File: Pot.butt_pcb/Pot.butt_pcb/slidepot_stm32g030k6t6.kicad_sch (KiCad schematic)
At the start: 11 parts, among them J3 Conn_01x05_Male, SW10 SW_Push, U2 STM32G030K6T6

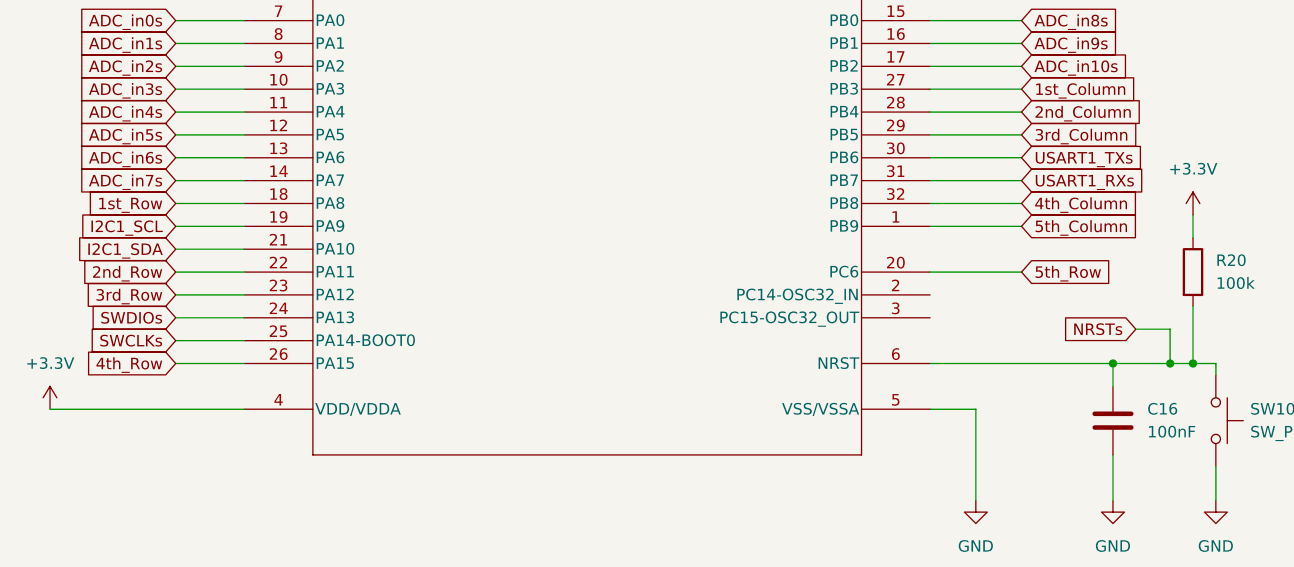
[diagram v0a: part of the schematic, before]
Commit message: Pot.but_pcb in progress
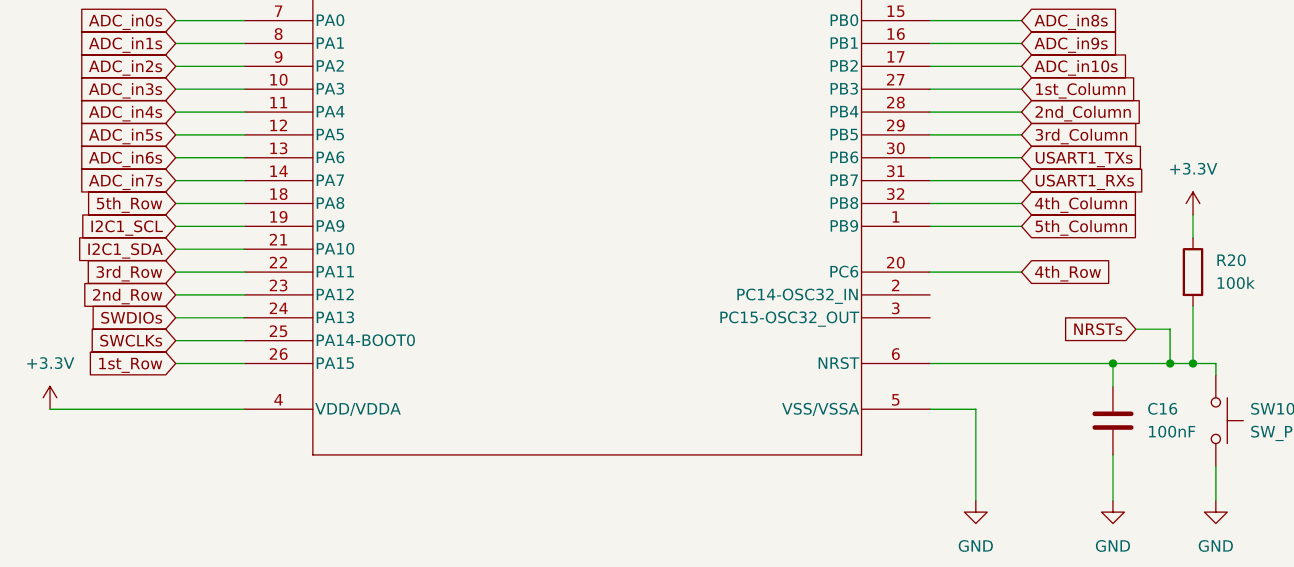
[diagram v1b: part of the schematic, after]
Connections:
- net 1st_Row: now also U2.26 (PA15); no longer U2.18 (PA8)
- net 2nd_Row: now also U2.23 (PA12); no longer U2.22 (PA11)
- net 3rd_Row: now also U2.22 (PA11); no longer U2.23 (PA12)
- net 4th_Row: now also U2.20 (PC6); no longer U2.26 (PA15)
- net 5th_Row: now also U2.18 (PA8); no longer U2.20 (PC6)
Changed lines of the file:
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@@
     )
   )
-  (global_label "4th_Row" (shape input) (at 49.53 83.82 180) (fields_autoplaced)
+  (global_label "1st_Row" (shape input) (at 49.53 83.82 180) (fields_autoplaced)
     (effects (font (size 1.27 1.27)) (justify right))
-    (property "Intersheet References" "${INTERSHEET_REFS}" (id 0) (at 39.3155 83.7406 0)
+    (property "Intersheet References" "${INTERSHEET_REFS}" (id 0) (at 39.4364 83.7406 0)
       (effects (font (size 1.27 1.27)) (justify right) hide)
     )
@@
     )
   )
-  (global_label "2nd_Row" (shape input) (at 49.53 73.66 180) (fields_autoplaced)
+  (global_label "3rd_Row" (shape input) (at 49.53 73.66 180) (fields_autoplaced)
     (effects (font (size 1.27 1.27)) (justify right))
-    (property "Intersheet References" "${INTERSHEET_REFS}" (id 0) (at 38.8921 73.5806 0)
+    (property "Intersheet References" "${INTERSHEET_REFS}" (id 0) (at 39.255 73.5806 0)
       (effects (font (size 1.27 1.27)) (justify right) hide)
     )
@@
     )
   )
-  (global_label "1st_Row" (shape input) (at 49.53 66.04 180) (fields_autoplaced)
+  (global_label "5th_Row" (shape input) (at 49.53 66.04 180) (fields_autoplaced)
     (effects (font (size 1.27 1.27)) (justify right))
-    (property "Intersheet References" "${INTERSHEET_REFS}" (id 0) (at 39.4364 65.9606 0)
+    (property "Intersheet References" "${INTERSHEET_REFS}" (id 0) (at 39.3155 65.9606 0)
       (effects (font (size 1.27 1.27)) (justify right) hide)
     )
@@
     )
   )
-  (global_label "5th_Row" (shape input) (at 143.51 73.66 0) (fields_autoplaced)
+  (global_label "4th_Row" (shape input) (at 143.51 73.66 0) (fields_autoplaced)
     (effects (font (size 1.27 1.27)) (justify left))
     (property "Intersheet References" "${INTERSHEET_REFS}" (id 0) (at 153.7245 73.5806 0)
@@
     )
   )
-  (global_label "3rd_Row" (shape input) (at 49.53 76.2 180) (fields_autoplaced)
+  (global_label "2nd_Row" (shape input) (at 49.53 76.2 180) (fields_autoplaced)
     (effects (font (size 1.27 1.27)) (justify right))
-    (property "Intersheet References" "${INTERSHEET_REFS}" (id 0) (at 39.255 76.1206 0)
+    (property "Intersheet References" "${INTERSHEET_REFS}" (id 0) (at 38.8921 76.1206 0)
       (effects (font (size 1.27 1.27)) (justify right) hide)
     )
